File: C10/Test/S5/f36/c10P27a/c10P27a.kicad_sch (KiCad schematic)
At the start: 5 parts

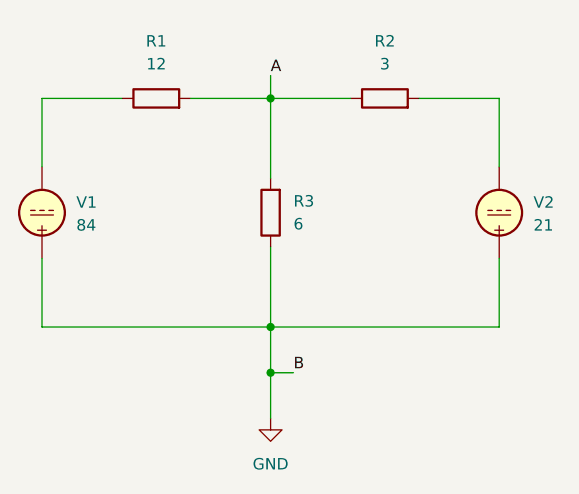
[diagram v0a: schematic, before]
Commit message: additiona upload Chapter 10
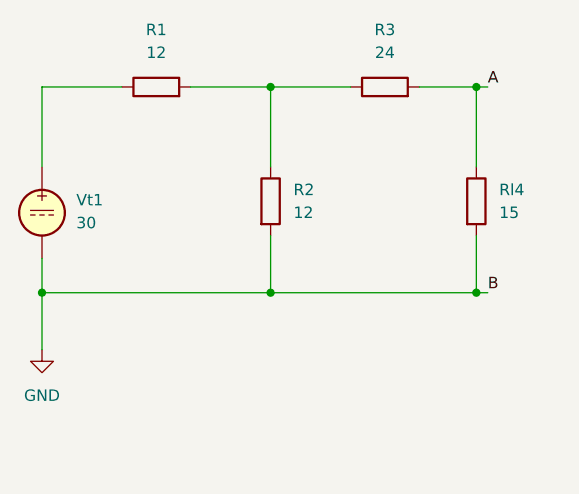
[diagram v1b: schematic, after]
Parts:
- removed V1: 84, symbol Simulation_SPICE:VDC
- removed V2: 21, symbol Simulation_SPICE:VDC
- added Rl4: 15, symbol Device:R
- added Vt1: 30, symbol Simulation_SPICE:VDC
- R2: value 3 -> 12
- R3: value 6 -> 24
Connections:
- net A: now also Rl4.1; no longer R1.2, R2.1
- net GND: now also R2.2, Rl4.2, Vt1.2; no longer R3.1
- net at R1.1: now also Vt1.1
- new net: R1.2, R2.1, R3.1
